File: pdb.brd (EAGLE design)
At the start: 50 x 100 mm, 50 parts, among them J1 XT60PWFEMALE, Q1 IRFR5305PBF, Q2 IRFR5305PBF, Q3 20MHz, U1 TSR_1-2433, U2 TXB0104, U3 ATMEGA48-20AU, U4 LTC2946CMSPBF, U5 LTC2946CMSPBF, U6 LTC2946CMSPBF, U7 AT30TS74SS8M

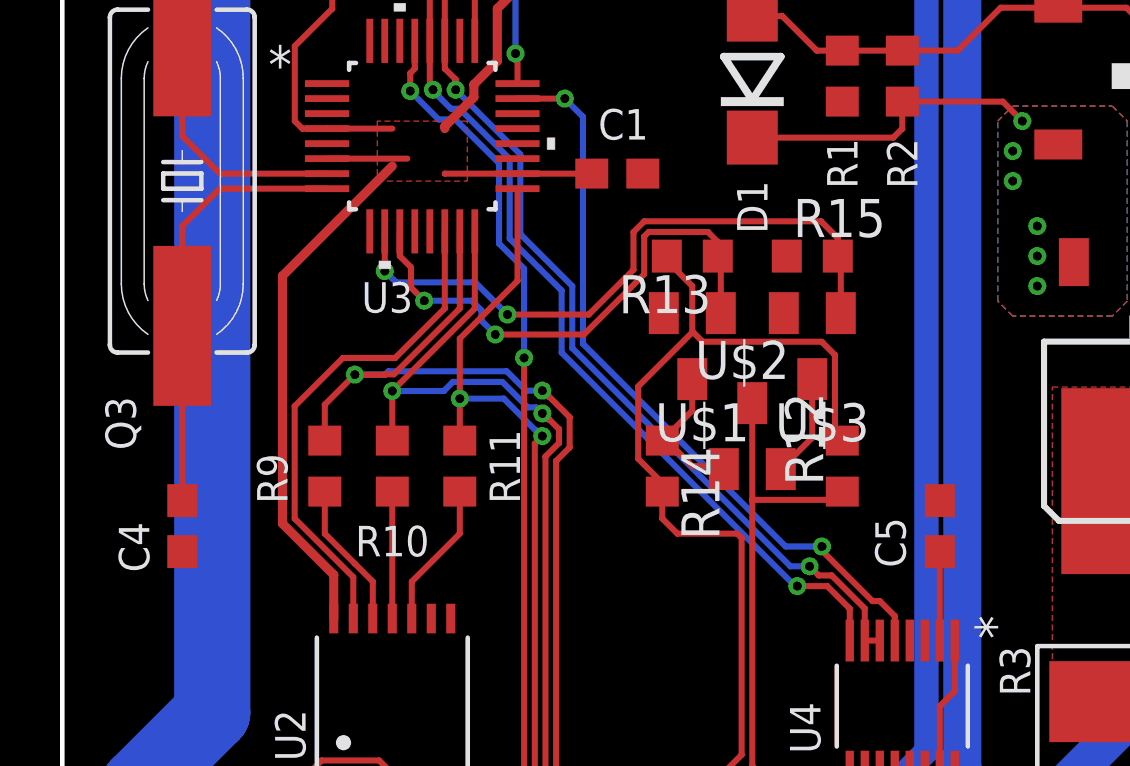
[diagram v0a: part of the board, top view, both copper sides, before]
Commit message: silkscreen
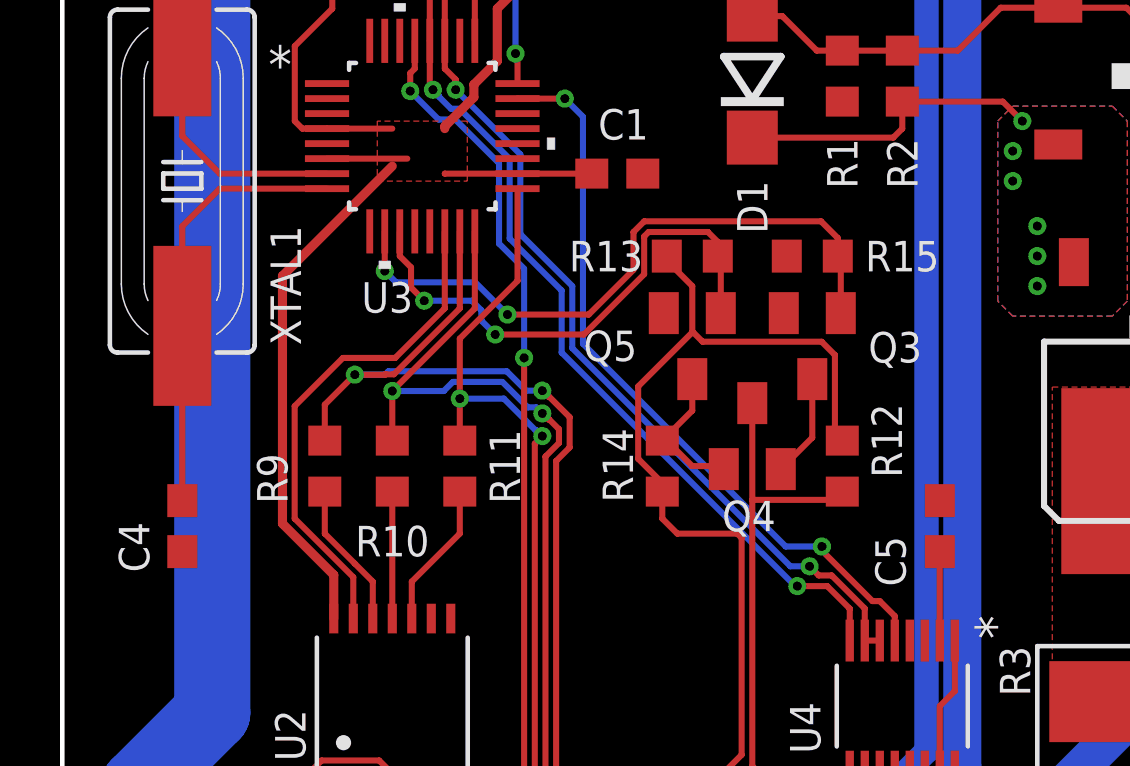
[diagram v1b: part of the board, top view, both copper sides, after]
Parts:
- removed U$3: BSN20,215, jonas_mosfet:BSN20_215
- added XTAL1: 20MHz, crystal:HC49UP
- Q3: value 20MHz -> BSN20,215; device crystal:HC49UP -> jonas_mosfet:BSN20_215
- moved Q3 21.7 mm to (25.0, 35.0), turned to 180 degrees
- renumbered U$1 to Q4, U$2 to Q5
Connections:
- net GND: now also Q3.2; no longer U$3.2
- net N$11: now also Q3.3; no longer U$3.3
- net N$27: now also XTAL1.2; no longer Q3.2
- net N$28: now also XTAL1.1; no longer Q3.1
- net RST_H: now also Q3.1; no longer U$3.1
